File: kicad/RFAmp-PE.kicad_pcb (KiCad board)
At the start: 2 copper layers, 62.2 x 34.2 mm, 29 parts, among them J1 Conn_01x03_Pin, J2 Conn_Coaxial_Small, J3 Conn_Coaxial_Small, J4 Conn_01x03_Pin, J5 Conn_01x02_Pin, Q1 BF961, Q2 2N7000

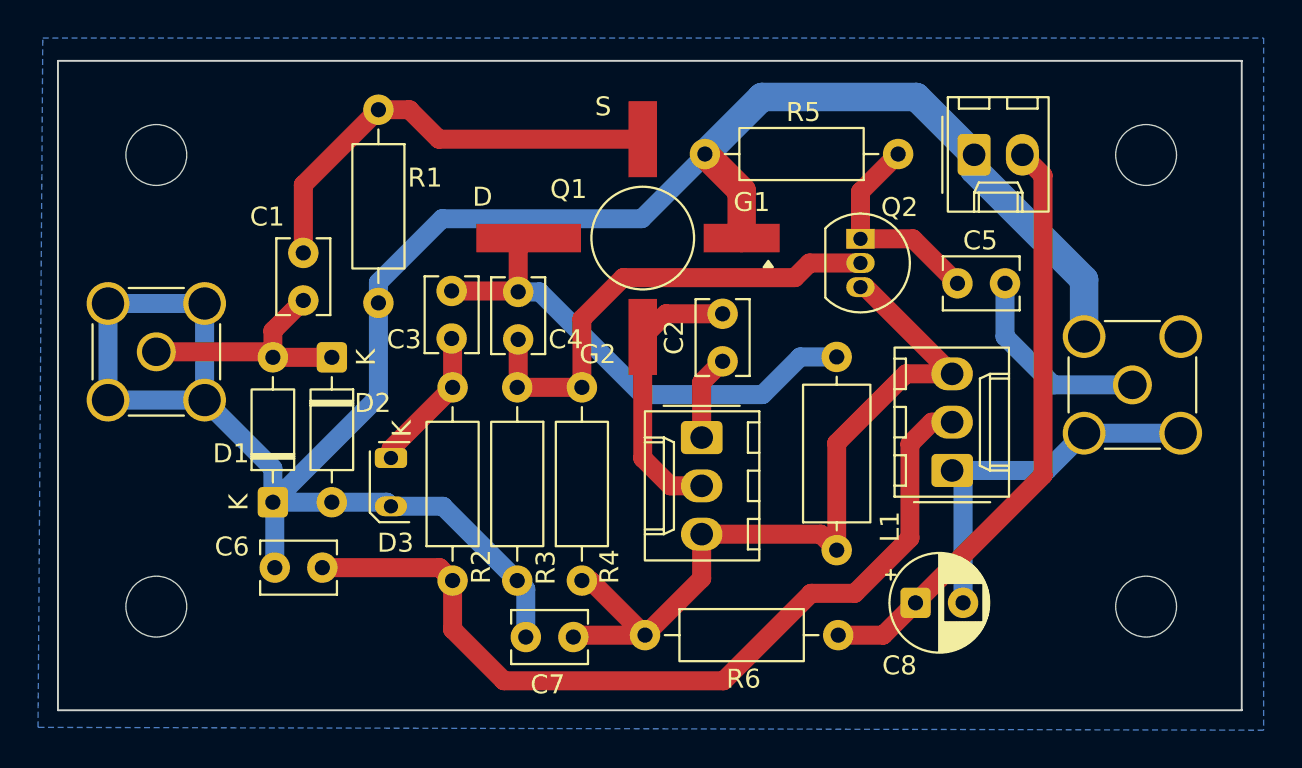
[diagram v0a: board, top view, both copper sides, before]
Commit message: V1.0 complete
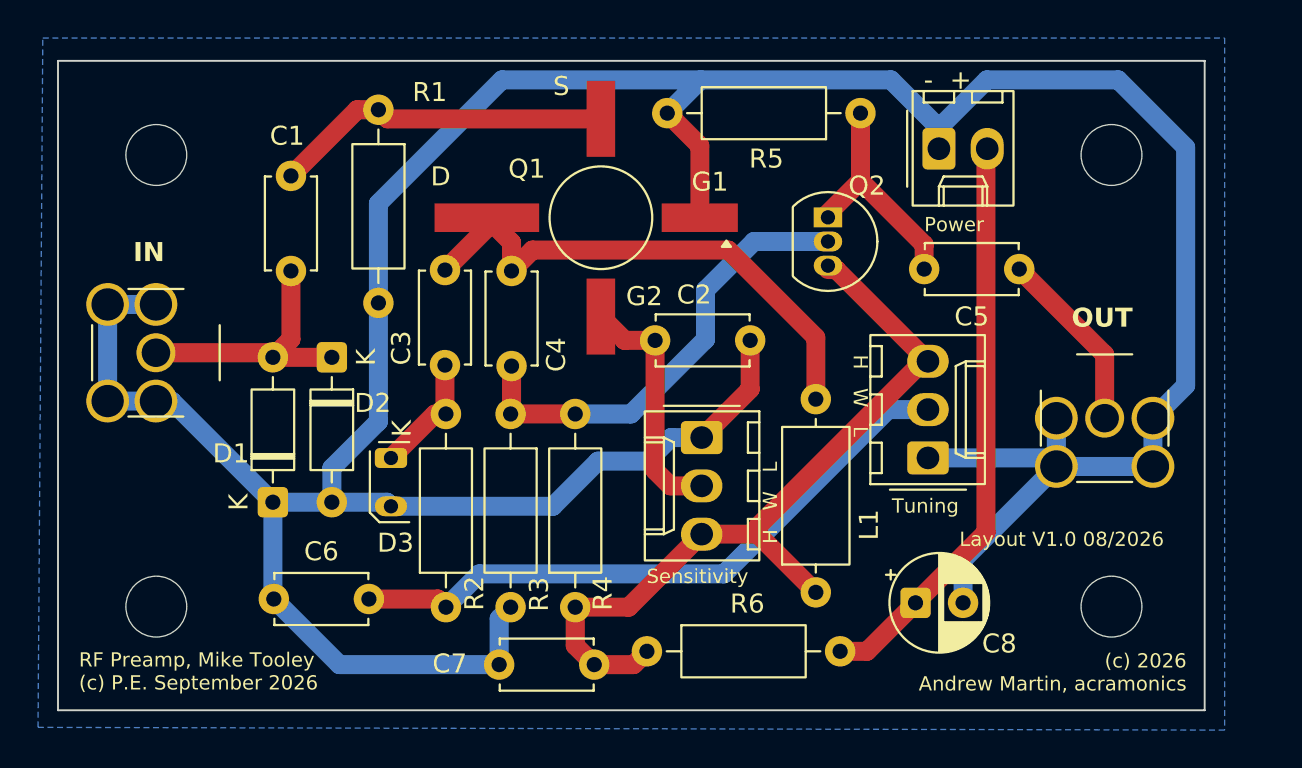
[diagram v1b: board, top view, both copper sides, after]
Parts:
- C1, C2, C3, C4, C5, C6, C7: footprint Capacitor_THT:C_Disc_D3.8mm_W2.6mm_P2.50mm -> Capacitor_THT:C_Disc_D4.7mm_W2.5mm_P5.00mm
- J2, J3: footprint Connector_Coaxial:SMA_Amphenol_901-144_Vertical -> ACRM:SMA_Vertical_AliExpress
- moved C1 4.10 mm to (46.0, 78.3)
- moved R5 2.92 mm to (75.9, 75.0)
- moved L1 2.48 mm to (73.5, 100.2)
- moved Q1 2.45 mm to (61.9, 80.5)
- moved J3 2.28 mm to (88.7, 91.0), turned to 90 degrees
- moved Q2 2.05 mm to (74.2, 80.5)
- moved C7 2.02 mm to (56.9, 104.0)
- moved J5 1.88 mm to (80.0, 76.9)
- moved C2 1.82 mm to (70.1, 87.0), turned to 180 degrees
- moved REF** 1.82 mm to (89.1, 101.0)
- moved REF** 1.82 mm to (89.1, 77.2)
- moved C6 1.65 mm to (45.0, 100.5)
- moved C3 1.44 mm to (54.0, 88.2)
- moved R2 1.44 mm to (54.1, 101.0)
- moved R4 1.44 mm to (60.9, 101.0)
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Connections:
- C2 pad 1: Net-(J1-Pin_1) -> GNDPWR
- J1 pad 1: Net-(J1-Pin_1) -> GNDPWR
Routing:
- net GNDPWR: track 136.1 -> 186.9 mm
- net Net-(J4-Pin_2): track 45.6 -> 33.9 mm
- net Net-(Q1-S): track 23.7 -> 17.9 mm
- net Net-(J1-Pin_1): track 4.47 -> 0.00 mm
- net Net-(Q1-D): track 26.4 -> 28.6 mm
- net Net-(J1-Pin_2): track 14.8 -> 13.0 mm
- net Net-(D1-A): track 13.0 -> 14.3 mm
- net Net-(D3-K): track 7.65 -> 6.44 mm
- net Net-(J5-Pin_2): track 31.6 -> 30.5 mm
- net Net-(Q2-G): track 25.4 -> 24.5 mm
- net Net-(J3-In): track 10.6 -> 9.70 mm
- net Net-(Q2-S): track 11.3 -> 12.0 mm
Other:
- board size 62.2 x 34.2 mm -> 60.3 x 34.2 mm
- board text added: "(c) 2026 Andrew Martin, acramonics"
- board text added: "- +"
- board text added: "H W L"
- board text added: "IN"
- board text added: "Layout V1.0 08/2026"
- board text added: "OUT"
- board text added: "Power"
- board text added: "RF Preamp, Mike Tooley (c) P.E. September 2026"
- board text added: "Sensitivity"
- board text added: "Tuning"
